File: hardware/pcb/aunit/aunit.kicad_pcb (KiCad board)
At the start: 2 copper layers, 62.2 x 21.6 mm, 48 parts, among them J1 BUS, J2 Input A, J3 Input B, J4 Control, J5 Flags, J6 Power, U1 74HC283, U2 74HC283, U3 74HC86, U4 74HC86, U5 74HC86, U6 74HC08, U7 74HC245, U8 74HC125

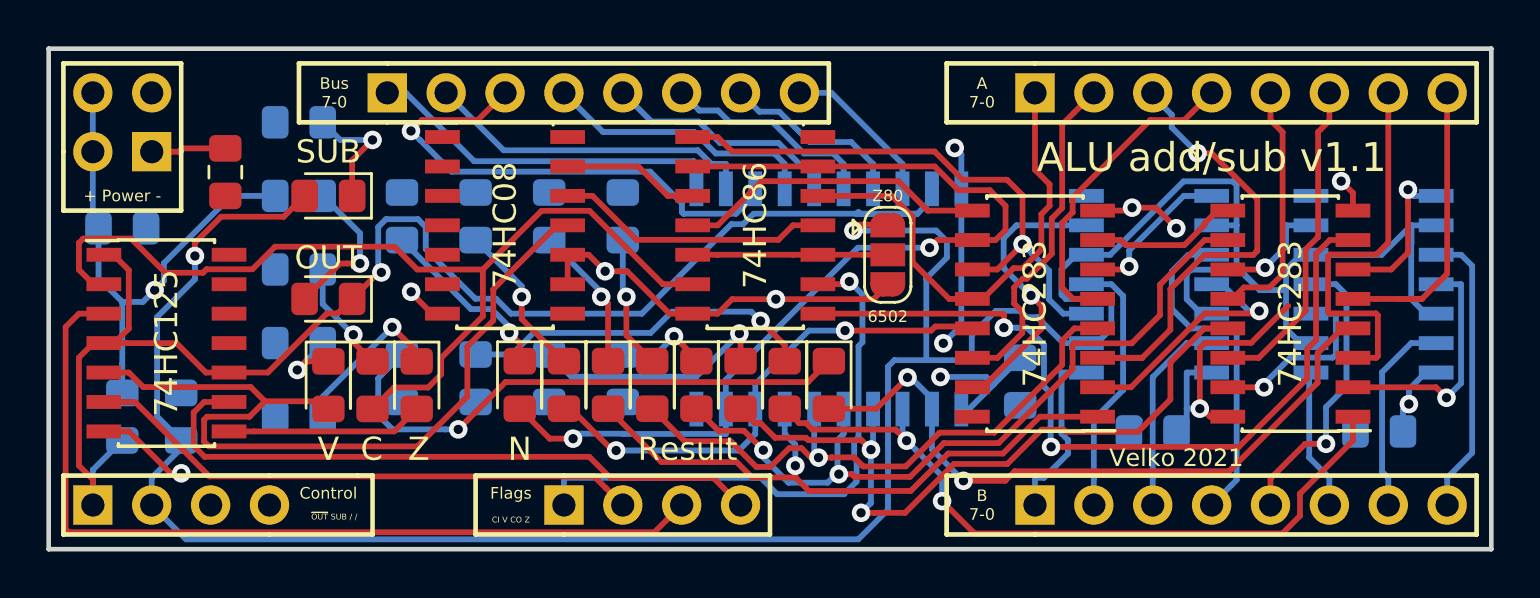
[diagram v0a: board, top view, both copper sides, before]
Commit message: Remove all tracks
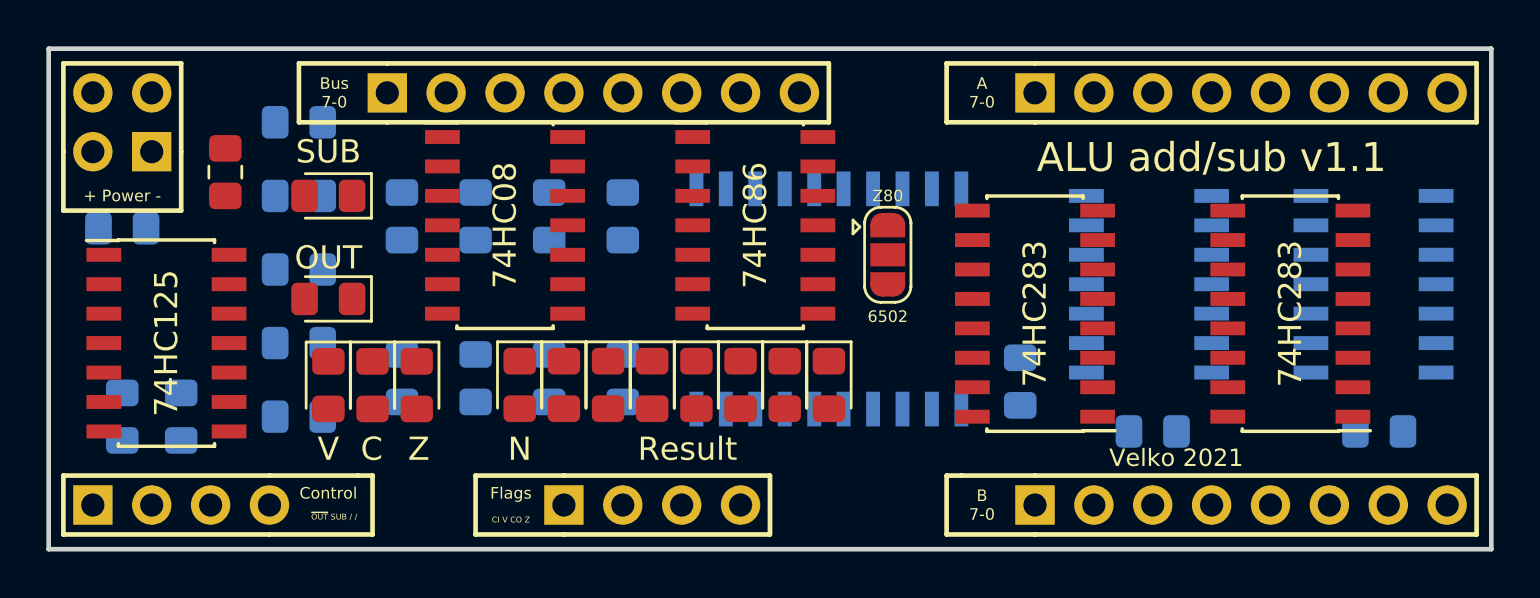
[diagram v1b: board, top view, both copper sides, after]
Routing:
- net ADD_SUB: track 123.7 -> 0.00 mm, vias 2 -> 0
- net ~OUT~: track 64.2 -> 0.00 mm, vias 1 -> 0
- net VCC: track 55.1 -> 0.00 mm, vias 6 -> 0
- net SUM7: track 42.4 -> 0.00 mm, vias 2 -> 0
- net CARRYD: track 41.7 -> 0.00 mm
- net COUT: track 37.7 -> 0.00 mm
- net OVFD: track 36.0 -> 0.00 mm
- net /CII: track 34.8 -> 0.00 mm, vias 2 -> 0
- net SUM3: track 33.3 -> 0.00 mm, vias 2 -> 0
- net GND: track 32.3 -> 0.00 mm, vias 7 -> 0
- net SUM1: track 32.1 -> 0.00 mm, vias 2 -> 0
- net SUM2: track 31.7 -> 0.00 mm, vias 2 -> 0
- net SUM0: track 29.8 -> 0.00 mm, vias 2 -> 0
- net ZIN: track 27.8 -> 0.00 mm
- net SUM5: track 26.8 -> 0.00 mm, vias 1 -> 0
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- removed copper zone on B.Cu, net GND
- removed copper zone on F.Cu, net VCC
